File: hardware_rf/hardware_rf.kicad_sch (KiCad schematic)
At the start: 93 parts, among them IC1 CC1125RHBR, IC2 BALF-SPI2-02D3, IC3 4259-63, IC4 4259-63, J1 Conn_Coaxial, J2 Conn_01x03_Socket, J3 Conn_02x20_Top_Bottom, J4 USB_C_Receptacle_USB2.0_16P, SW1 SW_Push, U1 RP2350A-QFN60, U2 W25Q128JVS, U3 GSQ5111, U4 SK5129, U5 AMS1117s-3.3, Y1 Crystal_GND24, Y2 Crystal_GND24

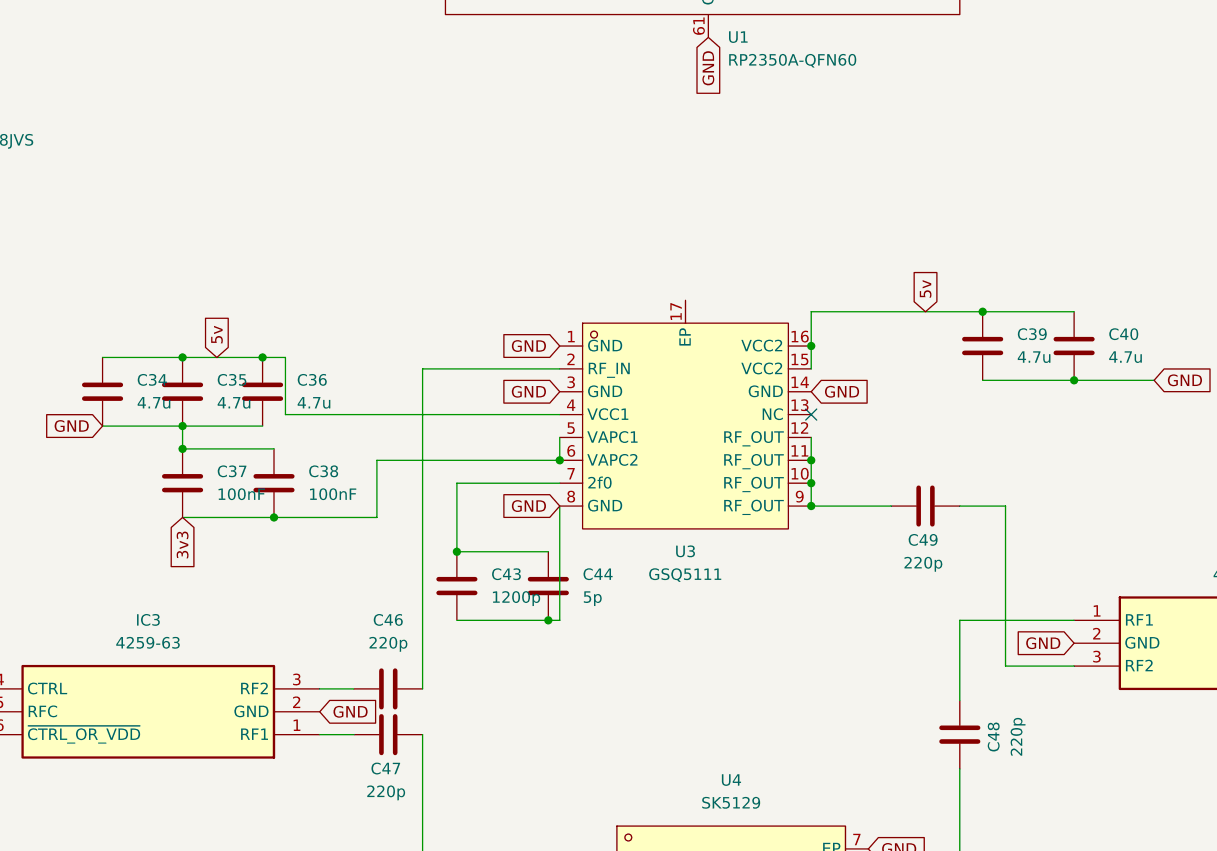
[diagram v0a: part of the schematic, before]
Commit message: Update PA
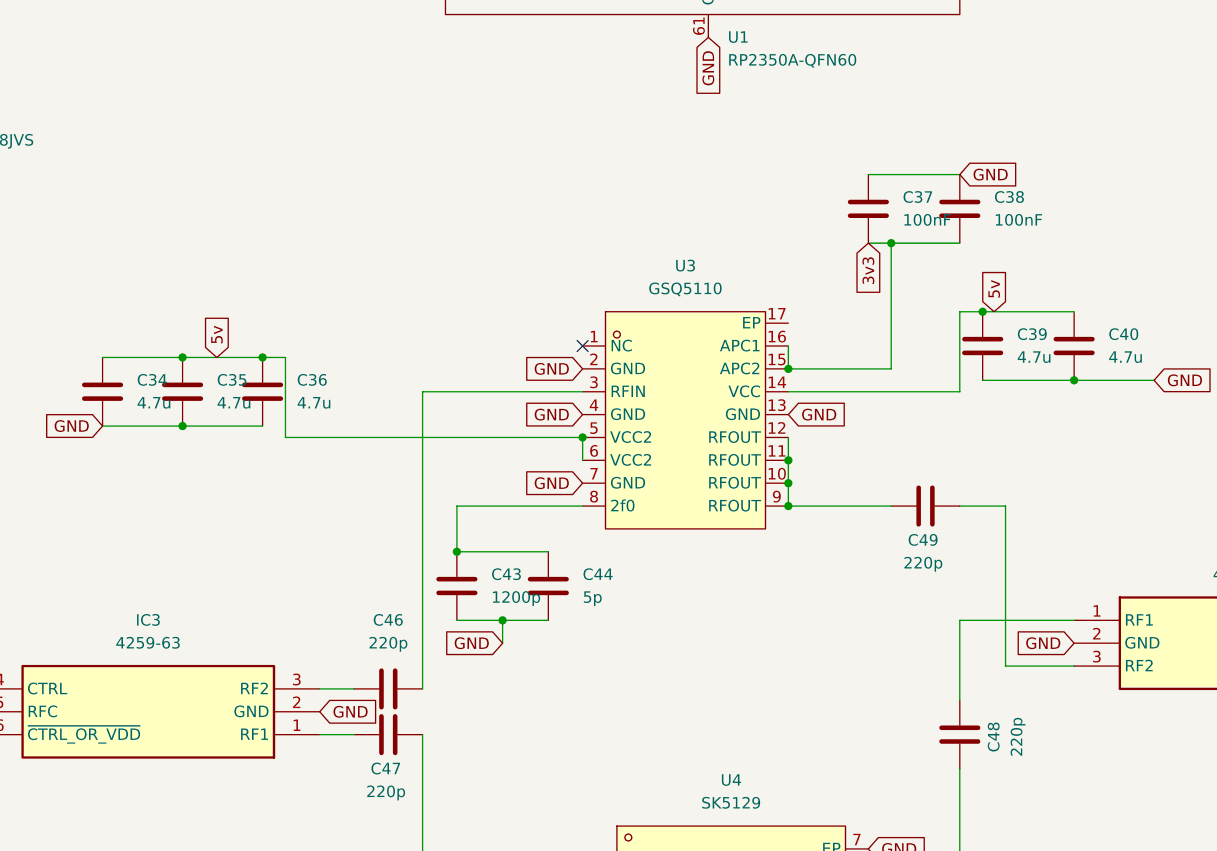
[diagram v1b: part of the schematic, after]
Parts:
- removed U3: GSQ5111, easyeda2kicad:QFN-16_L3.0-W3.0-P0.50-TL-EP1.65, symbol easyeda2kicad:GSQ5111
- added U3: GSQ5110, easyeda2kicad:QFN-16_L3.0-W3.0-P0.50-TL-EP2.0, symbol easyeda2kicad:GSQ5110
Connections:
- net 3v3: now also U3.15 (APC2), U3.16 (APC1)
- net 5v: now also U3.14 (VCC), U3.5 (VCC2), U3.6 (VCC2)
- net GND: now also U3.13 (GND), U3.2 (GND), U3.4 (GND), U3.7 (GND)
- net at C43.1, C44.1: now also U3.8 (2f0)
- net at C46.2: now also U3.3 (RFIN)
- net at C49.1: now also U3.10 (RFOUT), U3.11 (RFOUT), U3.12 (RFOUT), U3.9 (RFOUT)
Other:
- moved on the sheet: C37, C38
